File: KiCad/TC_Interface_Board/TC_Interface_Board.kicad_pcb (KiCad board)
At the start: 2 copper layers, 30 parts, among them J10 Conn_01x05, J11 Conn_01x05, J1_24V_ROW1 Conn_01x04, J1_CN1_24V1 Conn_01x03, J2_CN2_9V_Main1 Conn_01x02, J3_CN3_9V_Main1 Conn_01x02, J4 Conn_01x05, J5 Conn_01x05, J6 Conn_01x05, J7 Conn_01x05, J8 Conn_01x05, J9 Conn_01x05, Q1 DTC143E, Q2 DTC143E, U1 MC34063AP

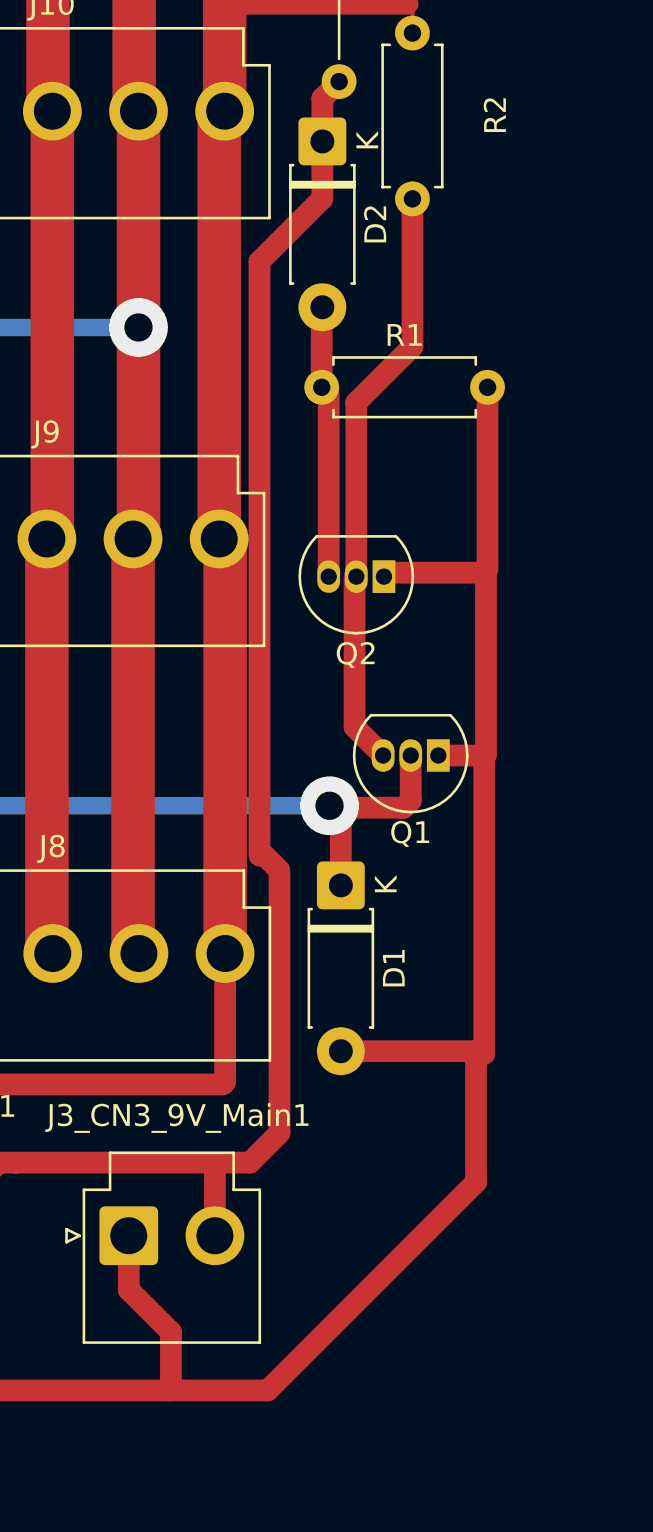
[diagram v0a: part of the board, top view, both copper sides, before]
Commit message: UPDATE
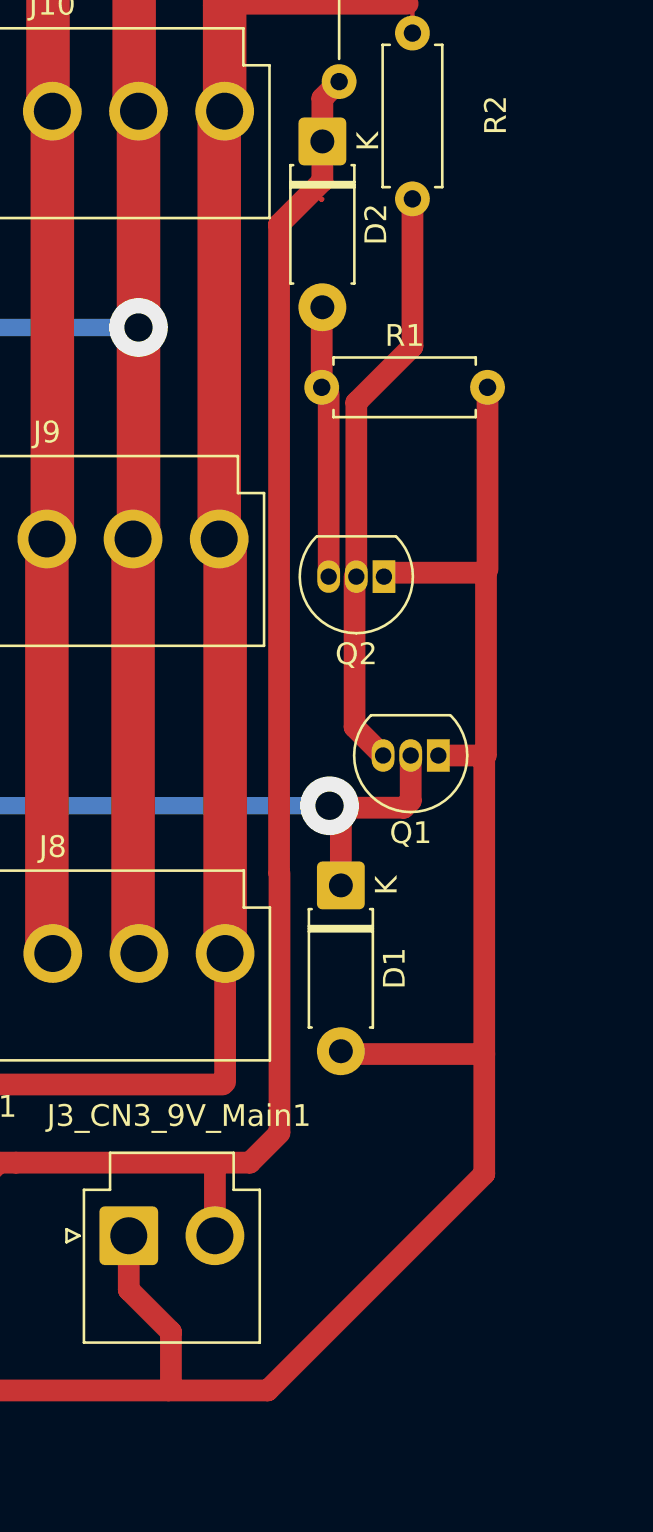
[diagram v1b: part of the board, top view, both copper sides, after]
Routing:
- net Net-(D1-A): track 123.7 -> 121.5 mm
- net Net-(D2-K): track 72.1 -> 71.4 mm
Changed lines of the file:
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@@
-	)
-	(segment
-		(start 165.67 93.266428)
-		(end 165.67 90.62)
-		(width 1)
-		(layer "F.Cu")
-		(net 4)
 	)
 	(segment
@@
 	)
 	(segment
-		(start 162.78 96.136428)
-		(end 165.616428 93.3)
-		(width 1)
-		(layer "F.Cu")
-		(net 4)
-	)
-	(segment
-		(start 163.02 123.44)
-		(end 162.78 123.44)
-		(width 0.2)
+		(start 165.67 90.62)
+		(end 165.67 92.45)
+		(width 1)
 		(layer "F.Cu")
 		(net 4)
@@
 	)
 	(segment
-		(start 163.696428 124.116428)
-		(end 163.02 123.44)
-		(width 1)
-		(layer "F.Cu")
-		(net 4)
-	)
-	(segment
 		(start 147.4425 140.91)
 		(end 150.8025 137.55)
@@
 	)
 	(segment
+		(start 163.68 124.223572)
+		(end 163.7 124.243572)
+		(width 0.2)
+		(layer "F.Cu")
+		(net 4)
+	)
+	(segment
 		(start 160.7325 137.7125)
 		(end 160.69 137.67)
@@
 	)
 	(segment
+		(start 165.67 92.45)
+		(end 163.68 94.44)
+		(width 1)
+		(layer "F.Cu")
+		(net 4)
+	)
+	(segment
 		(start 163.696428 124.24)
 		(end 163.696428 124.116428)
@@
 	)
 	(segment
-		(start 162.78 123.44)
-		(end 162.78 96.136428)
-		(width 1)
-		(layer "F.Cu")
-		(net 4)
-	)
-	(segment
 		(start 160.7325 140.91)
 		(end 160.7325 137.7125)
@@
 	)
 	(segment
+		(start 163.68 94.44)
+		(end 163.68 124.223572)
+		(width 1)
+		(layer "F.Cu")
+		(net 4)
+	)
+	(segment
 		(start 160.69 137.67)
 		(end 160.81 137.55)
@@
 	)
 	(segment
-		(start 172.73 132.43)
-		(end 171.64 132.43)
-		(width 0.2)
-		(layer "F.Cu")
-		(net 8)
-	)
-	(segment
-		(start 172.73 132.43)
-		(end 166.52 132.43)
+		(start 166.84 132.56)
+		(end 166.71 132.43)
 		(width 1)
 		(layer "F.Cu")
@@
 	)
 	(segment
-		(start 158.6 148.02)
-		(end 163.16 148.02)
-		(width 1)
-		(layer "F.Cu")
-		(net 8)
-	)
-	(segment
 		(start 130.99 148.02)
 		(end 144.58 148.02)
@@
 	)
 	(segment
+		(start 173.11 132.56)
+		(end 166.84 132.56)
+		(width 1)
+		(layer "F.Cu")
+		(net 8)
+	)
+	(segment
 		(start 131.656428 144.52)
 		(end 131.6725 144.503928)
@@
 	)
 	(segment
+		(start 173.11 138.07)
+		(end 163.16 148.02)
+		(width 1)
+		(layer "F.Cu")
+		(net 8)
+	)
+	(segment
 		(start 172.99 118.84)
 		(end 171 118.84)
@@
 	)
 	(segment
-		(start 172.73 138.45)
-		(end 172.73 132.43)
-		(width 1)
-		(layer "F.Cu")
-		(net 8)
-	)
-	(segment
 		(start 144.58 148.02)
 		(end 158.6 148.02)
@@
 	)
 	(segment
-		(start 172.98 132.43)
-		(end 173.11 132.56)
-		(width 0.2)
-		(layer "F.Cu")
-		(net 8)
-	)
-	(segment
 		(start 130.99 145.203572)
 		(end 130.966428 145.18)
@@
 	)
 	(segment
-		(start 163.16 148.02)
-		(end 172.73 138.45)
-		(width 1)
-		(layer "F.Cu")
-		(net 8)
-	)
-	(segment
 		(start 131.6725 144.503928)
 		(end 131.6725 141)
@@
 	)
 	(segment
+		(start 166.71 132.43)
+		(end 166.52 132.43)
+		(width 1)
+		(layer "F.Cu")
+		(net 8)
+	)
+	(segment
 		(start 173.19 118.81)
 		(end 173.19 110.52)
@@
 	)
 	(segment
+		(start 163.16 148.02)
+		(end 158.6 148.02)
+		(width 1)
+		(layer "F.Cu")
+		(net 8)
+	)
+	(segment
 		(start 173.19 110.52)
 		(end 173.11 110.44)
@@
 	)
 	(segment
-		(start 171.64 132.43)
-		(end 172.98 132.43)
-		(width 0.2)
-		(layer "F.Cu")
-		(net 8)
-	)
-	(segment
 		(start 131.626428 144.52)
 		(end 131.656428 144.52)
@@
 		(layer "F.Cu")
 		(net 8)
+	)
+	(segment
+		(start 173.11 138.07)
+		(end 173.11 132.56)
+		(width 1)
+		(layer "F.Cu")
+		(net 8)
